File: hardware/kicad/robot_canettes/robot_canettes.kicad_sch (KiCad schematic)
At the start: 0 parts

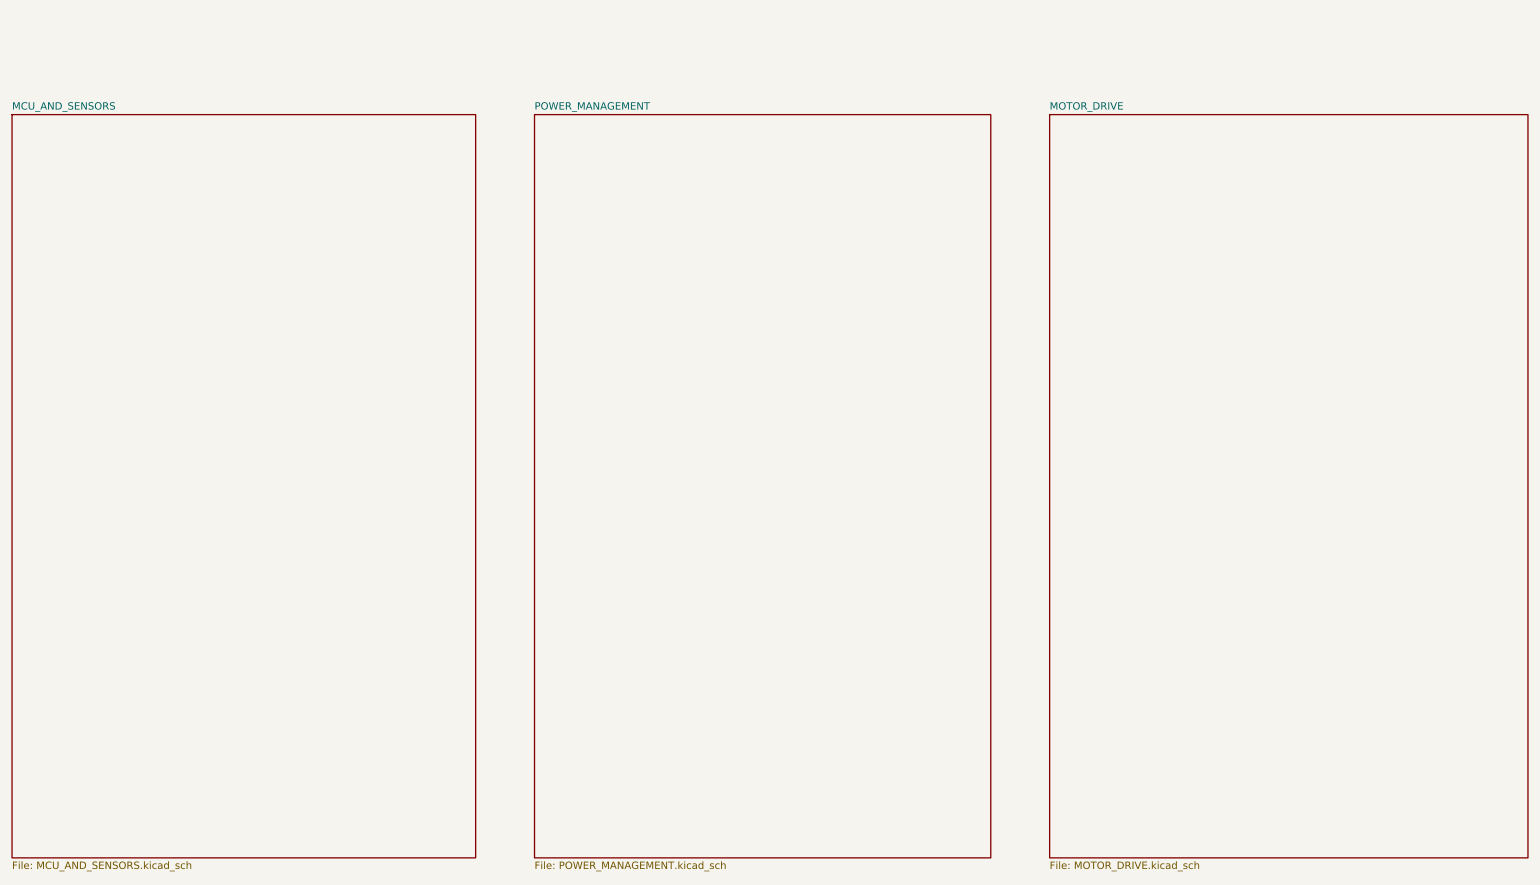
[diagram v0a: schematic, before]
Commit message: MOTOR_DRIVE
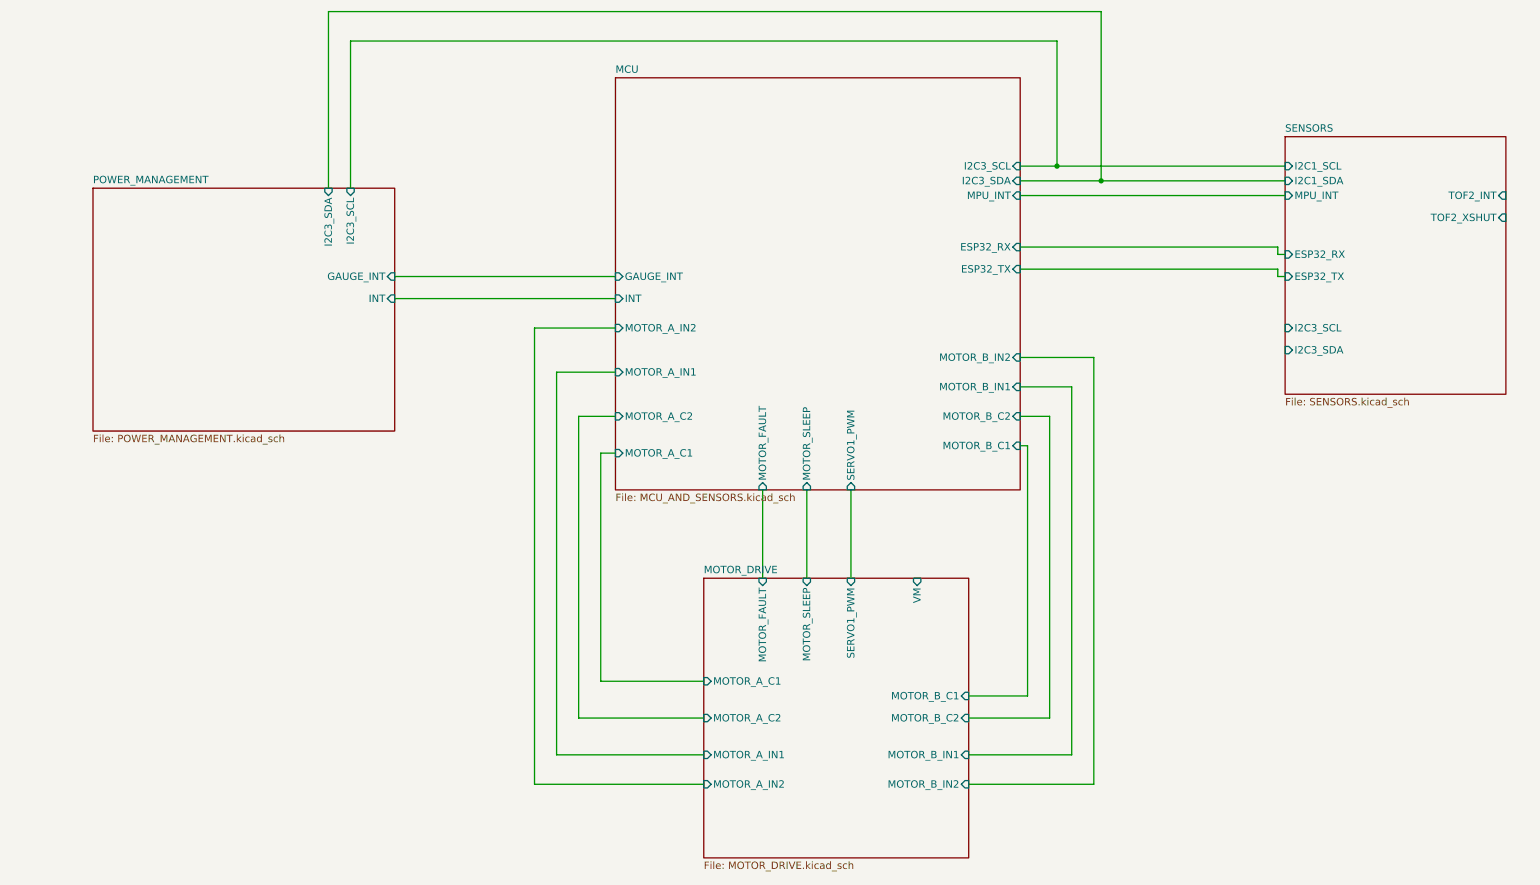
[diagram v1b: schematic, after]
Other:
- sheet MCU_AND_SENSORS renamed MCU
- added sheet SENSORS (SENSORS.kicad_sch)
- sheet MCU ports: added ESP32_RX, ESP32_TX, GAUGE_INT, I2C3_SCL, I2C3_SDA, INT, MOTOR_A_C1, MOTOR_A_C2, MOTOR_A_IN1, MOTOR_A_IN2, MOTOR_B_C1, MOTOR_B_C2, MOTOR_B_IN1, MOTOR_B_IN2, MOTOR_FAULT, MOTOR_SLEEP, MPU_INT, SERVO1_PWM; removed none
- sheet MOTOR_DRIVE ports: added MOTOR_A_C1, MOTOR_A_C2, MOTOR_A_IN1, MOTOR_A_IN2, MOTOR_B_C1, MOTOR_B_C2, MOTOR_B_IN1, MOTOR_B_IN2, MOTOR_FAULT, MOTOR_SLEEP, SERVO1_PWM, VM; removed none
- sheet POWER_MANAGEMENT ports: added GAUGE_INT, I2C3_SCL, I2C3_SDA, INT; removed none
